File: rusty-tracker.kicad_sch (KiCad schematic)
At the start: 176 parts, among them J1 SIM8051-6-0-14-01-X, J2 USB_C_Receptacle_USB2.0, J3 NFC, J4 tag-connect-swd, J5 Battery Connector, J6 Conn_01x01, J7 Conn_01x01, Q1 RUM002N02T2L, Q2 RUM002N02T2L, Q3 RUM002N02T2L, Q4 RUM002N02T2L, Q5 RUM002N02T2L, SW1 SW_Push, T1 Tab, T2 Tab, T3 Tab, T4 Tab, U1 uBLOX SARA-R42x, U10 MM8130-2600, U11 MM8130-2600, U12 MX25R1635F, U13 LSM6DS3, U14 LPS22HBTR, U2 nRF52840, U3 VC1034B018F, U5 MCP73833, U8 B39242B8328P810, U9 MM8130-2600, Y1 32 MHz, Y2 32.768 kHz

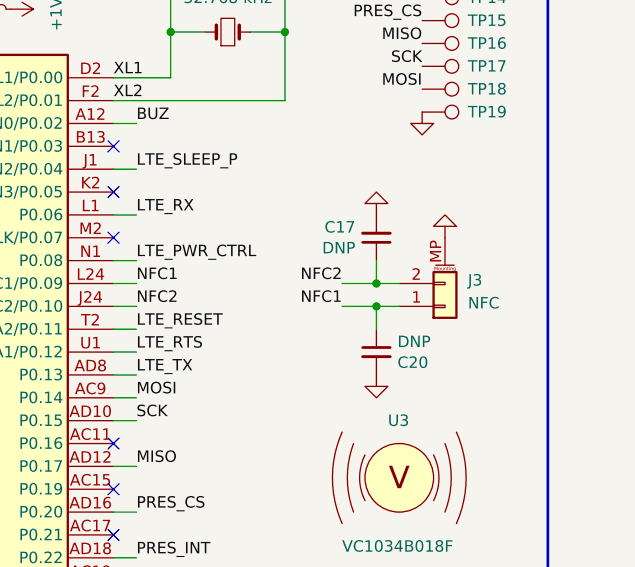
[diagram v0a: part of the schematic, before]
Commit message: Order sent to JLCPCB
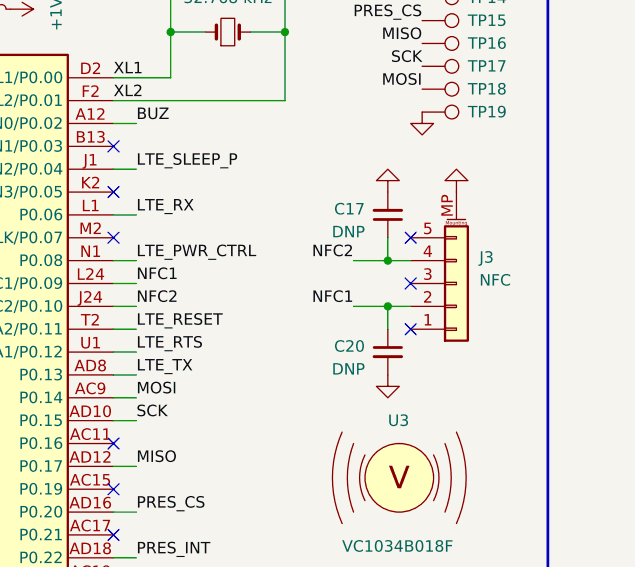
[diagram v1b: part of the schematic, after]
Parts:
- J3: footprint Connector_JST:JST_SH_SM02B-SRSS-TB_1x02-1MP_P1.00mm_Horizontal -> Connector_FFC-FPC:TE_0-1734839-5_1x05-1MP_P0.5mm_Horizontal; symbol Connector_Generic_MountingPin:Conn_01x02_MountingPin -> Connector_Generic_MountingPin:Conn_01x05_MountingPin
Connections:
- net NFC1: now also J3.2 (Pin_2); no longer J3.1 (Pin_1)
- net NFC2: now also J3.4 (Pin_4); no longer J3.2 (Pin_2)
- no-connect marks 57 -> 60
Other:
- moved on the sheet: C17, C20
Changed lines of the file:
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@@
   (junction (at 190.5 177.8) (diameter 0) (color 0 0 0 0)
   )
-  (junction (at 382.27 121.92) (diameter 0) (color 0 0 0 0)
+  (junction (at 383.54 119.38) (diameter 0) (color 0 0 0 0)
   )
   (junction (at 280.67 72.39) (diameter 0) (color 0 0 0 0)
@@
   (junction (at 173.99 165.1) (diameter 0) (color 0 0 0 0)
   )
-  (junction (at 382.27 124.46) (diameter 0) (color 0 0 0 0)
+  (junction (at 383.54 124.46) (diameter 0) (color 0 0 0 0)
   )
   (junction (at 173.99 222.25) (diameter 0) (color 0 0 0 0)
@@
   (no_connect (at 107.95 91.44))
   (no_connect (at 353.06 165.1))
+  (no_connect (at 386.08 121.92))
   (no_connect (at 142.24 252.73))
   (no_connect (at 50.8 227.33))
@@
   (no_connect (at 107.95 60.96))
   (no_connect (at 142.24 250.19))
+  (no_connect (at 386.08 116.84))
   (no_connect (at 68.58 227.33))
   (no_connect (at 287.02 205.74))
@@
   (no_connect (at 77.47 227.33))
   (no_connect (at 107.95 58.42))
+  (no_connect (at 386.08 127))
   (no_connect (at 64.77 62.23))
   (no_connect (at 24.13 227.33))
@@
     (stroke (width 0) (type default))
   )
-  (wire (pts (xy 382.27 124.46) (xy 382.27 127))
+  (wire (pts (xy 383.54 124.46) (xy 383.54 127))
     (stroke (width 0) (type default))
   )
@@
     (stroke (width 0) (type default))
   )
-  (wire (pts (xy 382.27 119.38) (xy 382.27 121.92))
+  (wire (pts (xy 383.54 116.84) (xy 383.54 119.38))
     (stroke (width 0) (type default))
   )
@@
     (stroke (width 0) (type default))
   )
-  (wire (pts (xy 378.46 124.46) (xy 382.27 124.46))
+  (wire (pts (xy 379.73 124.46) (xy 383.54 124.46))
     (stroke (width 0) (type default))
   )
@@
     (stroke (width 0) (type default))
   )
-  (wire (pts (xy 378.46 121.92) (xy 382.27 121.92))
+  (wire (pts (xy 379.73 119.38) (xy 383.54 119.38))
     (stroke (width 0) (type default))
   )
@@
     (stroke (width 0.3) (type default))
   )
-  (wire (pts (xy 382.27 121.92) (xy 384.81 121.92))
+  (wire (pts (xy 383.54 119.38) (xy 386.08 119.38))
     (stroke (width 0) (type default))
   )
@@
     (stroke (width 0) (type default))
   )
-  (wire (pts (xy 382.27 124.46) (xy 384.81 124.46))
+  (wire (pts (xy 383.54 124.46) (xy 386.08 124.46))
     (stroke (width 0) (type default))
   )
@@
     (effects (font (size 1.27 1.27)) (justify left bottom))
   )
-  (label "NFC1" (at 378.46 124.46 180) (fields_autoplaced)
+  (label "NFC1" (at 379.73 124.46 180) (fields_autoplaced)
     (effects (font (size 1.27 1.27)) (justify right bottom))
   )
@@
     (effects (font (size 1.27 1.27)) (justify right bottom))
   )
-  (label "NFC2" (at 378.46 121.92 180) (fields_autoplaced)
+  (label "NFC2" (at 379.73 119.38 180) (fields_autoplaced)
     (effects (font (size 1.27 1.27)) (justify right bottom))
   )
@@
     )
   )
-  (symbol (lib_id "power:GND") (at 382.27 114.3 0) (mirror x) (unit 1)
+  (symbol (lib_id "power:GND") (at 383.54 111.76 0) (mirror x) (unit 1)
     (in_bom yes) (on_board yes) (dnp no)
-    (property "Reference" "#PWR055" (at 382.27 107.95 0)
+    (property "Reference" "#PWR055" (at 383.54 105.41 0)
       (effects (font (size 1.27 1.27)) hide)
     )
-    (property "Value" "GND" (at 382.397 111.0488 90)
+    (property "Value" "GND" (at 383.667 108.5088 90)
       (effects (font (size 1.27 1.27)) (justify right) hide)
     )
-    (property "Footprint" "" (at 382.27 114.3 0)
+    (property "Footprint" "" (at 383.54 111.76 0)
       (effects (font (size 1.27 1.27)))
     )
-    (property "Datasheet" "" (at 382.27 114.3 0)
+    (property "Datasheet" "" (at 383.54 111.76 0)
       (effects (font (size 1.27 1.27)))
     )
@@
     )
   )
-  (symbol (lib_id "Device:C_Small") (at 382.27 129.54 0) (mirror y) (unit 1)
-    (in_bom yes) (on_board yes) (dnp no)
-    (property "Reference" "C20" (at 384.6068 130.7084 0)
-      (effects (font (size 1.27 1.27)) (justify right))
+  (symbol (lib_id "Device:C_Small") (at 383.54 129.54 0) (mirror y) (unit 1)
+    (in_bom yes) (on_board yes) (dnp no) (fields_autoplaced)
+    (property "Reference" "C20" (at 381 128.9113 0)
+      (effects (font (size 1.27 1.27)) (justify left))
     )
-    (property "Value" "DNP" (at 384.6068 128.397 0)
-      (effects (font (size 1.27 1.27)) (justify right))
+    (property "Value" "DNP" (at 381 131.4513 0)
+      (effects (font (size 1.27 1.27)) (justify left))
     )
-    (property "Footprint" "passive:C_0402" (at 382.27 129.54 0)
+    (property "Footprint" "passive:C_0402" (at 383.54 129.54 0)
       (effects (font (size 1.27 1.27)) hide)
     )
-    (property "Datasheet" "" (at 382.27 129.54 0)
+    (property "Datasheet" "" (at 383.54 129.54 0)
       (effects (font (size 1.27 1.27)))
     )
-    (property "Tolerance" "" (at 382.27 129.54 0)
+    (property "Tolerance" "" (at 383.54 129.54 0)
       (effects (font (size 1.524 1.524)) hide)
     )
-    (property "Manufacturer" "" (at 528.32 309.88 0)
+    (property "Manufacturer" "" (at 529.59 309.88 0)
       (effects (font (size 1.524 1.524)) hide)
     )
-    (property "MFPN" "" (at 382.27 129.54 0)
+    (property "MFPN" "" (at 383.54 129.54 0)
       (effects (font (size 1.27 1.27)) hide)
     )
-    (property "Comment" "C0G,50V" (at 382.27 129.54 0)
+    (property "Comment" "C0G,50V" (at 383.54 129.54 0)
       (effects (font (size 1.27 1.27)) hide)
     )
@@
     )
   )
-  (symbol (lib_id "power:GND") (at 382.27 132.08 0) (mirror y) (unit 1)
+  (symbol (lib_id "power:GND") (at 383.54 132.08 0) (mirror y) (unit 1)
     (in_bom yes) (on_board yes) (dnp no)
-    (property "Reference" "#PWR059" (at 382.27 138.43 0)
+    (property "Reference" "#PWR059" (at 383.54 138.43 0)
       (effects (font (size 1.27 1.27)) hide)
     )
-    (property "Value" "GND" (at 382.143 135.3312 90)
+    (property "Value" "GND" (at 383.413 135.3312 90)
       (effects (font (size 1.27 1.27)) (justify right) hide)
     )
-    (property "Footprint" "" (at 382.27 132.08 0)
+    (property "Footprint" "" (at 383.54 132.08 0)
       (effects (font (size 1.27 1.27)))
     )
-    (property "Datasheet" "" (at 382.27 132.08 0)
+    (property "Datasheet" "" (at 383.54 132.08 0)
       (effects (font (size 1.27 1.27)))
     )
@@
     )
   )
-  (symbol (lib_id "power:GND") (at 389.89 116.84 180) (unit 1)
+  (symbol (lib_id "power:GND") (at 391.16 111.76 180) (unit 1)
     (in_bom yes) (on_board yes) (dnp no) (fields_autoplaced)
-    (property "Reference" "#PWR061" (at 389.89 110.49 0)
+    (property "Reference" "#PWR061" (at 391.16 105.41 0)
       (effects (font (size 1.27 1.27)) hide)
     )
-    (property "Value" "GND" (at 389.763 113.5888 90)
+    (property "Value" "GND" (at 391.033 108.5088 90)
       (effects (font (size 1.27 1.27)) (justify right) hide)
     )
-    (property "Footprint" "" (at 389.89 116.84 0)
+    (property "Footprint" "" (at 391.16 111.76 0)
       (effects (font (size 1.27 1.27)) hide)
     )
-    (property "Datasheet" "" (at 389.89 116.84 0)
+    (property "Datasheet" "" (at 391.16 111.76 0)
       (effects (font (size 1.27 1.27)) hide)
     )
@@
     )
   )
-  (symbol (lib_id "Device:C_Small") (at 382.27 116.84 0) (mirror x) (unit 1)
-    (in_bom yes) (on_board yes) (dnp no)
-    (property "Reference" "C17" (at 379.9332 115.6716 0)
+  (symbol (lib_id "Device:C_Small") (at 383.54 114.3 0) (mirror x) (unit 1)
+    (in_bom yes) (on_board yes) (dnp no) (fields_autoplaced)
+    (property "Reference" "C17" (at 381 113.6586 0)
       (effects (font (size 1.27 1.27)) (justify right))
     )
-    (property "Value" "DNP" (at 379.9332 117.983 0)
+    (property "Value" "DNP" (at 381 116.1986 0)
       (effects (font (size 1.27 1.27)) (justify right))
     )
-    (property "Footprint" "passive:C_0402" (at 382.27 116.84 0)
+    (property "Footprint" "passive:C_0402" (at 383.54 114.3 0)
       (effects (font (size 1.27 1.27)) hide)
     )
-    (property "Datasheet" "" (at 382.27 116.84 0)
+    (property "Datasheet" "" (at 383.54 114.3 0)
       (effects (font (size 1.27 1.27)))
     )
-    (property "Tolerance" "" (at 382.27 116.84 0)
+    (property "Tolerance" "" (at 383.54 114.3 0)
       (effects (font (size 1.524 1.524)) hide)
     )
-    (property "Manufacturer" "" (at 236.22 -63.5 0)
+    (property "Manufacturer" "" (at 237.49 -66.04 0)
       (effects (font (size 1.524 1.524)) hide)
     )
-    (property "MFPN" "" (at 382.27 116.84 0)
+    (property "MFPN" "" (at 383.54 114.3 0)
       (effects (font (size 1.27 1.27)) hide)
     )
-    (property "Comment" "C0G,50V" (at 382.27 116.84 0)
+    (property "Comment" "C0G,50V" (at 383.54 114.3 0)
       (effects (font (size 1.27 1.27)) hide)
     )
@@
     )
   )
-  (symbol (lib_id "Connector_Generic_MountingPin:Conn_01x02_MountingPin") (at 389.89 124.46 0) (mirror x) (unit 1)
+  (symbol (lib_id "Connector_Generic_MountingPin:Conn_01x05_MountingPin") (at 391.16 121.92 0) (mirror x) (unit 1)
     (in_bom yes) (on_board yes) (dnp no) (fields_autoplaced)
-    (property "Reference" "J3" (at 392.43 121.5643 0)
+    (property "Reference" "J3" (at 393.7 119.0243 0)
       (effects (font (size 1.27 1.27)) (justify left))
     )
-    (property "Value" "NFC" (at 392.43 124.1043 0)
+    (property "Value" "NFC" (at 393.7 121.5643 0)
       (effects (font (size 1.27 1.27)) (justify left))
     )
-    (property "Footprint" "Connector_JST:JST_SH_SM02B-SRSS-TB_1x02-1MP_P1.00mm_Horizontal" (at 389.89 124.46 0)
+    (property "Footprint" "Connector_FFC-FPC:TE_0-1734839-5_1x05-1MP_P0.5mm_Horizontal" (at 391.16 121.92 0)
       (effects (font (size 1.27 1.27)) hide)
     )
-    (property "Datasheet" "~" (at 389.89 124.46 0)
+    (property "Datasheet" "~" (at 391.16 121.92 0)
       (effects (font (size 1.27 1.27)) hide)
     )
-    (property "MFPN" "SM02B-SRSS-TB(LF)(SN)" (at 389.89 124.46 0)
+    (property "MFPN" "SM02B-SRSS-TB(LF)(SN)" (at 391.16 121.92 0)
       (effects (font (size 1.27 1.27)) hide)
     )
     (pin "1")
     (pin "2")
+    (pin "3")
+    (pin "4")
+    (pin "5")
     (pin "MP")
     (instances
